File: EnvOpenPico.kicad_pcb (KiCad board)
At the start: 2 copper layers, 21 x 51.3 mm, 26 parts, among them J1 USB_B_Micro, J2 Conn_01x02, J3 Conn_02x18_Odd_Even, J4 Conn_02x18_Odd_Even, J5 Conn_01x03_Male, U1 NCP1117-3.3_SOT223, U2 W25Q16JVSSIQ, U3 RP2040, Y1 ABLS-12.000MHZ-B4-T

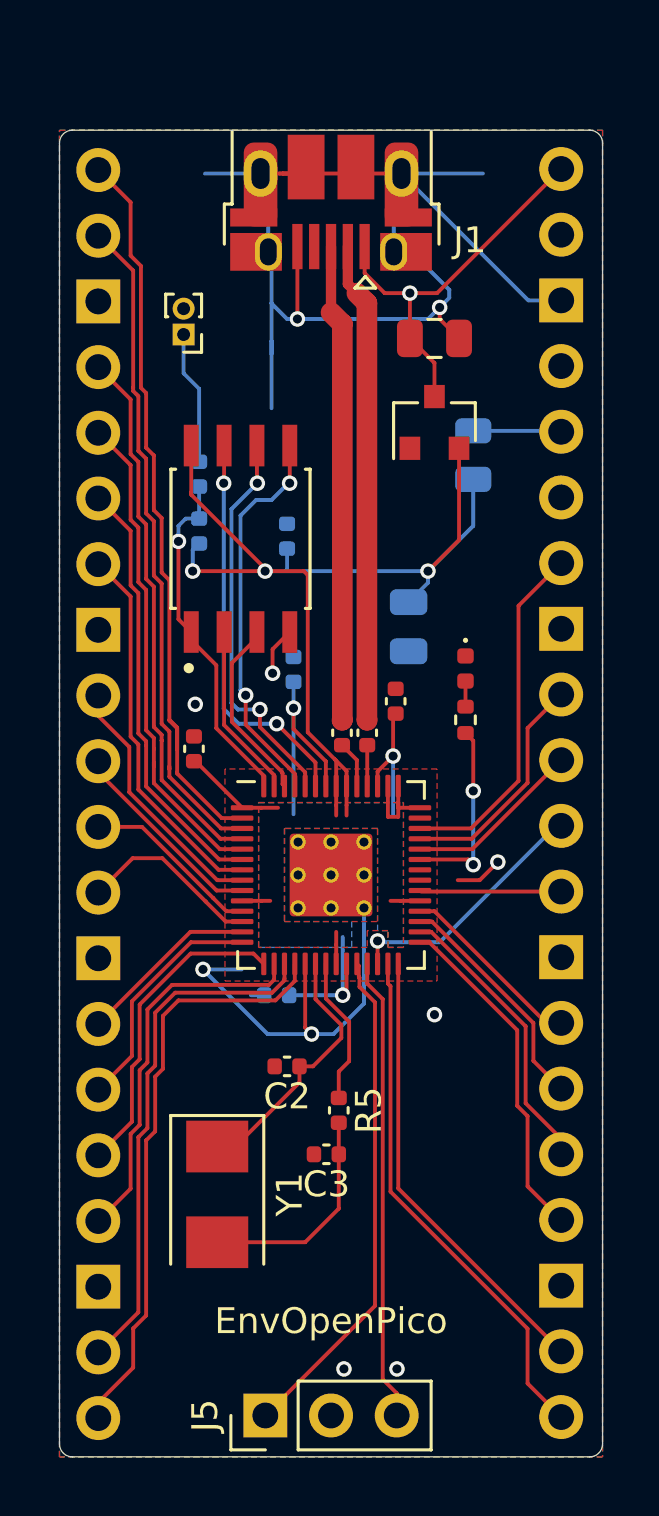
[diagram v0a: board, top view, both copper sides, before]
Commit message: Redesign
I need sleep.
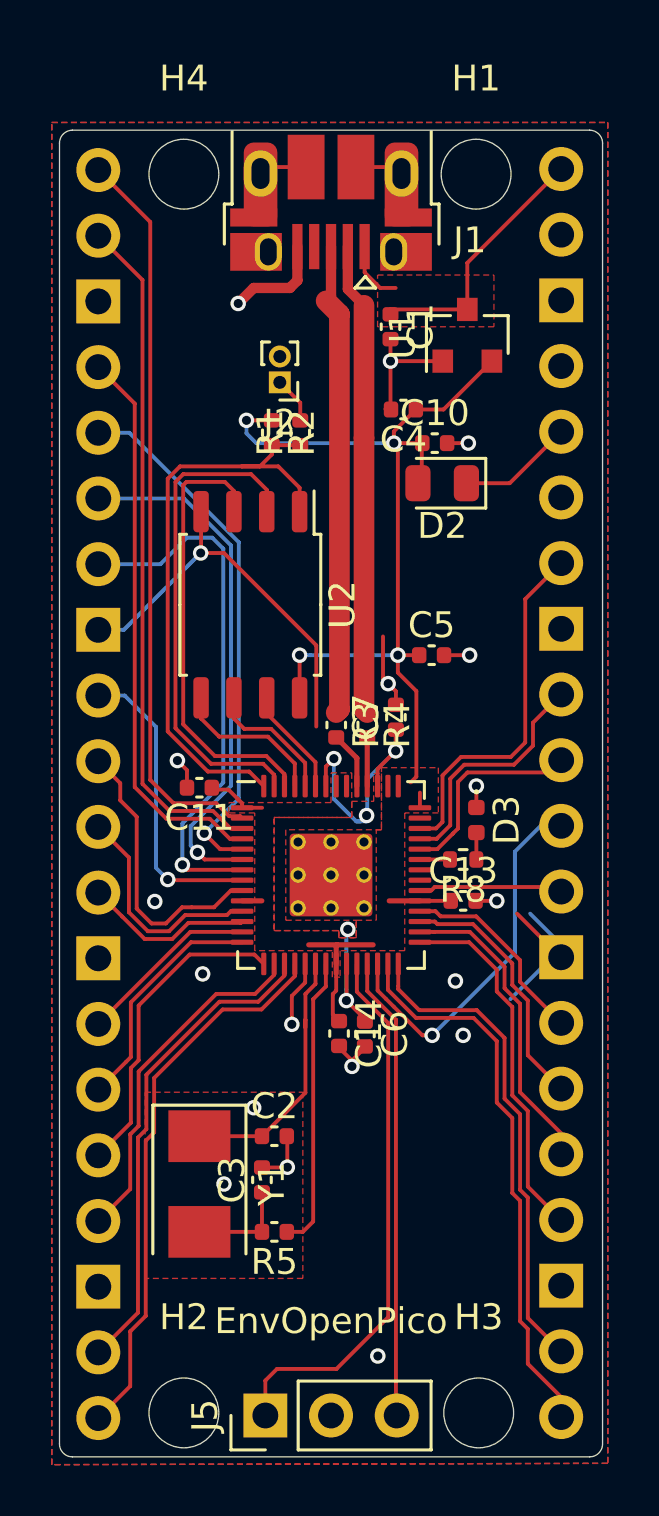
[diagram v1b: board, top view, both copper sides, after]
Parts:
- removed C8: 1u, Capacitor_SMD:C_0402_1005Metric
- added C10: 1u, Capacitor_SMD:C_0402_1005Metric, F.Cu at (94.1, 60.8)
- added C13: 100n, Capacitor_SMD:C_0402_1005Metric, F.Cu at (95.2, 78.5)
- added C14: 100n, Capacitor_SMD:C_0402_1005Metric, F.Cu at (90.4, 83.6)
- added H1: MountingHole, MountingHole:MountingHole_2.7mm_M2.5, F.Cu at (95.7, 50.4)
- added H2: MountingHole, MountingHole:MountingHole_2.7mm_M2.5, F.Cu at (84.4, 98.3)
- added H3: MountingHole, MountingHole:MountingHole_2.7mm_M2.5, F.Cu at (95.8, 98.3)
- added H4: MountingHole, MountingHole:MountingHole_2.7mm_M2.5, F.Cu at (84.4, 50.4)
- C1: footprint Capacitor_SMD:C_0805_2012Metric -> Capacitor_SMD:C_0402_1005Metric
- C4: footprint Capacitor_SMD:C_0805_2012Metric -> Capacitor_SMD:C_0402_1005Metric; moved to F.Cu
- C5, C7, D2, R1, R2: moved to F.Cu
- U2: footprint W25Q16JVSSIQ:SOIC127P790X216-8N -> Package_SO:SOIC-8_5.23x5.23mm_P1.27mm
- moved C6 12.9 mm to (91.4, 83.7), turned to 270 degrees
- moved C4 8.40 mm to (92.9, 59.5), turned to 180 degrees
- moved C5 7.24 mm to (94.0, 69.0), turned to 0 degrees
- moved D3 5.88 mm to (95.7, 75.4)
- moved R8 5.40 mm to (95.2, 76.9), turned to 180 degrees
- moved R5 5.32 mm to (87.9, 91.3), turned to 180 degrees
- moved R2 4.73 mm to (87.8, 60.4), turned to 270 degrees
- moved C7 4.37 mm to (92.6, 71.4)
- moved R1 4.22 mm to (88.9, 60.4)
- moved J2 4.15 mm to (88.1, 58.5)
- moved U1 3.60 mm to (95.4, 56.6)
- moved C2 2.74 mm to (87.9, 87.6), turned to 0 degrees
- moved C3 2.68 mm to (87.4, 89.3), turned to 90 degrees
- moved U2 2.58 mm to (87.0, 67.0), turned to 270 degrees
- moved C1 1.76 mm to (92.4, 56.3), turned to 270 degrees
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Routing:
- net GND: track 70.5 -> 50.0 mm, vias 10 -> 19
- net /QSPI_SD1: track 6.76 -> 19.3 mm
- net /QSPI_SD3: track 15.5 -> 4.19 mm, vias 2 -> 0
- net /QSPI_SD2: track 7.20 -> 17.4 mm
- net /QSPI_SS: track 13.6 -> 23.7 mm, vias 1 -> 0
- net /QSPI_SCLK: track 15.3 -> 5.16 mm, vias 2 -> 0
- net /QSPI_SD0: track 15.2 -> 6.02 mm, vias 2 -> 0
- net /GPIO25: track 7.35 -> 1.16 mm, vias 2 -> 0
- net +3V3: track 53.2 -> 47.1 mm, vias 3 -> 4
- net /GPIO5: track 14.7 -> 20.7 mm, vias 0 -> 1
- net /XOUT: track 5.72 -> 11.4 mm
- net /RUN: track 9.87 -> 14.6 mm
- net Net-(C3-Pad1): track 8.48 -> 4.05 mm
- net +1V1: track 19.6 -> 15.7 mm, vias 3 -> 5
- net /GPIO4: track 16.8 -> 20.4 mm, vias 0 -> 1
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- added copper zone on F.Cu, net +1V1
- added copper zone on F.Cu, net VBUS
- removed copper zone on B.Cu, net +1V1
